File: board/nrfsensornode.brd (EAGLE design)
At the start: 40.3 x 34.3 mm, 16 parts, among them IC1 LM1117MPX-3.3, IC2 DS1820

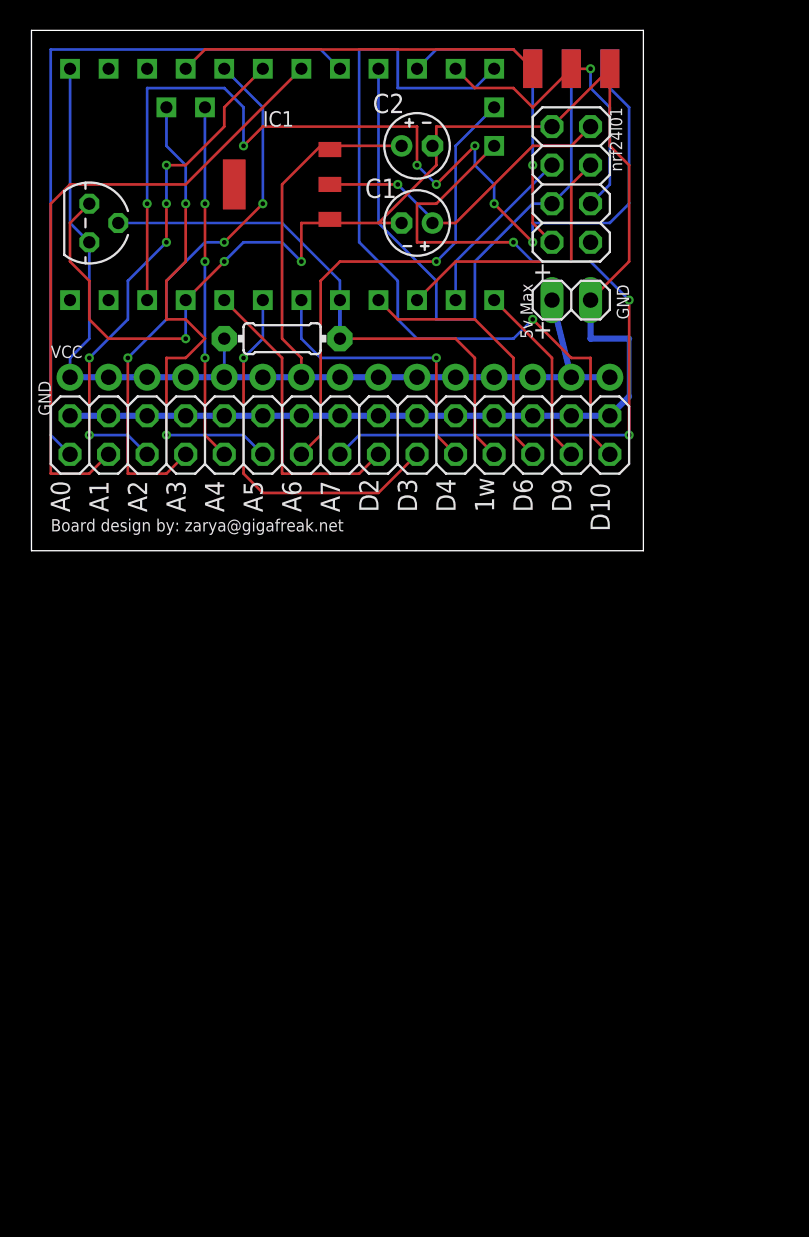
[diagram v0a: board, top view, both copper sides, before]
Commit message: Updates
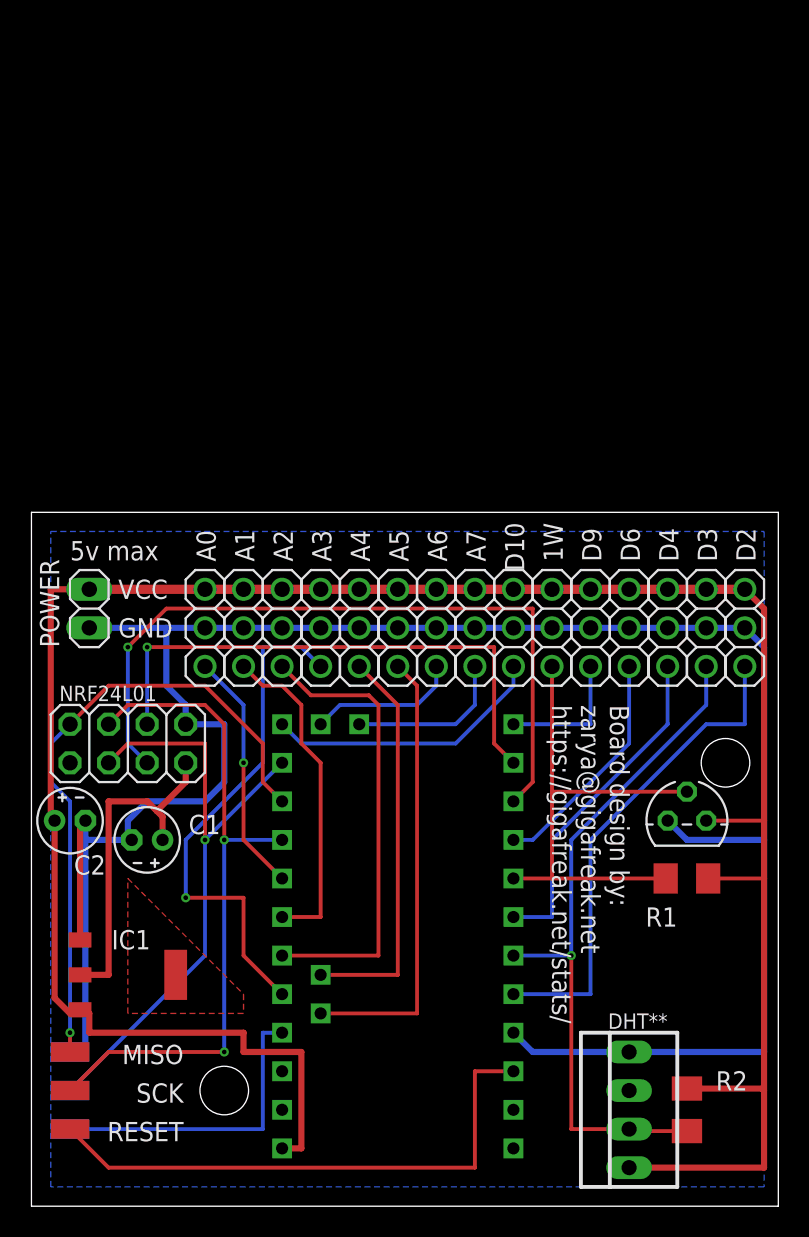
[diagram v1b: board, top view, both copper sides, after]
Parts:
- removed JP1: (no value), pinhead:1X02
- removed JP3: (no value), pinhead:2X04
- removed JP4: (no value), pinhead:2X15
- removed PAD1, PAD2, PAD3, PAD4, PAD5, PAD6: WIREPADSMD1,27-254, wirepad:SMD1,27-2,54
- removed VCC: (no value), adafruit:1X15-CB
- added 1W, A0, A1, A2, A3, A4, A5, A6, A7, D10, D2, D3, D4, D6, D9: (no value), adafruit:1X03
- added 5V, GND, MISO, MOSI, RESET, SCK: WIREPADSMD1,27-254, wirepad:SMD1,27-2,54
- added DHT**: 22-23-2041, con-molex:22-23-2041
- added NRF24L01: (no value), pinhead:2X04
- added POWER: (no value), pinhead:1X02
- added R2: 4.7k, adafruit:M1206
- added U$2: (no value), adafruit:OSHWLOGO_TOL_0.2
- IC1: value LM1117MPX-3.3 -> (none)
- IC2: value DS1820 -> DS18b20
- R1: device adafruit:0204/7 -> adafruit:M1206
- moved IC2 55.7 mm to (43.2, 25.4), turned to 0 degrees
- moved IC1 53.1 mm to (6.35, 15.2), turned to 270 degrees
- moved U$1 50.1 mm to (24.1, 17.8), turned to 180 degrees
- moved C2 50.0 mm to (2.54, 25.4)
- moved R1 44.5 mm to (43.2, 21.6), turned to 180 degrees
- moved C1 44.4 mm to (7.62, 24.1)
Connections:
- new net IC1COOL: IC1.4
- net +3V3: now also NRF24L01.2; no longer JP3.2
- net +5V: now also 5V.1; no longer PAD4.1
- net A0: now also A0.1; no longer JP4.1
- net A1: now also A1.1; no longer JP4.3
- net A2: now also A2.1; no longer JP4.5
- net A3: now also A3.1; no longer JP4.7
- net A4: now also A4.1; no longer JP4.9
- net A5: now also A5.1; no longer JP4.11
- net A6: now also A6.1; no longer JP4.13
- net A7: now also A7.1; no longer JP4.15
- net D10: now also D10.1; no longer JP4.29
- net D2: now also D2.1; no longer JP4.17
- net D3: now also D3.1, DHT**.2, R2.2; no longer JP4.19
- net D4: now also D4.1; no longer JP4.21
- net D5: now also 1W.1; no longer JP4.23
- net D6: now also D6.1; no longer JP4.25
- net D7: now also NRF24L01.4; no longer JP3.4
- net D8: now also NRF24L01.3; no longer JP3.3
- net D9: now also D9.1; no longer JP4.27
- net GND: now also 1W.2, A0.2, A1.2, A2.2, A3.2, A4.2, A5.2, A6.2, A7.2, D10.2, D2.2, D3.2, D4.2, D6.2, D9.2, DHT**.4, GND.1, NRF24L01.1, POWER.2; no longer JP1.2, JP3.1, JP4.10, JP4.12, JP4.14, JP4.16, JP4.18, JP4.2, JP4.20, JP4.22, JP4.24, JP4.26, JP4.28, JP4.30, JP4.4, JP4.6, JP4.8, PAD6.1
- net MISO: now also MISO.1, NRF24L01.7; no longer JP3.7, PAD1.1
- net MOSI: now also MOSI.1, NRF24L01.6; no longer JP3.6, PAD5.1
- net RAW: now also 1W.3, A0.3, A1.3, A2.3, A3.3, A4.3, A5.3, A6.3, A7.3, D10.3, D2.3, D3.3, D4.3, D6.3, D9.3, DHT**.1, POWER.1, R2.1; no longer JP1.1, VCC.1, VCC.10, VCC.11, VCC.12, VCC.13, VCC.14, VCC.15, VCC.2, VCC.3, VCC.4, VCC.5, VCC.6, VCC.7, VCC.8, VCC.9
- net RESET: now also RESET.1; no longer PAD3.1
- net SCK: now also NRF24L01.5, SCK.1; no longer JP3.5, PAD2.1
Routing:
- net RAW: track 86.9 -> 160.4 mm
- net A7: track 53.2 -> 10.7 mm, vias 3 -> 0
- net D10: track 52.5 -> 18.6 mm, vias 1 -> 0
- net RESET: track 68.8 -> 36.6 mm, vias 7 -> 0
- net D7: track 18.1 -> 49.1 mm, vias 0 -> 1
- net A0: track 46.8 -> 16.1 mm, vias 0 -> 1
- net D8: track 11.5 -> 36.1 mm, vias 0 -> 1
- net GND: track 121.3 -> 145.2 mm, vias 3 -> 0
- net A6: track 31.8 -> 9.94 mm, vias 1 -> 0
- net MISO: track 20.6 -> 42.3 mm
- net D3: track 25.0 -> 45.6 mm
- net A1: track 42.3 -> 21.9 mm
- net MOSI: track 20.9 -> 40.6 mm
- net D2: track 19.9 -> 32.4 mm
- net SCK: track 40.5 -> 45.3 mm, vias 0 -> 2
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- added copper zone on layer 16, net GND
- added copper zone on layer 1, net IC1COOL
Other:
- board size 40.3 x 34.3 mm -> 49.2 x 45.7 mm
- board text added: "5v max"
- board text added: "Board design by: zarya@gigafreak.net https://gigafreak.net/stats/"
- board text added: "NrfSensorNode v1"
- board text removed: "+"
- board text removed: "1w"
- board text removed: "5v Max"
- board text removed: "A0"
- board text removed: "A1"
- board text removed: "A2"
- board text removed: "A3"
- board text removed: "A4"
- board text removed: "A5"
- board text removed: "A6"
- board text removed: "A7"
- board text removed: "Board design by: zarya@gigafreak.net"
- board text removed: "D10"
- board text removed: "D2"
- board text removed: "D3"
- board text removed: "D4"
- board text removed: "D6"
- board text removed: "D9"
- board text removed: "IC1"
- board text removed: "https://gigafreak.net/stats/"
- board text removed: "nrf24l01"
